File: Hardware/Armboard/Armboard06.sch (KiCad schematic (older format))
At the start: 7 parts

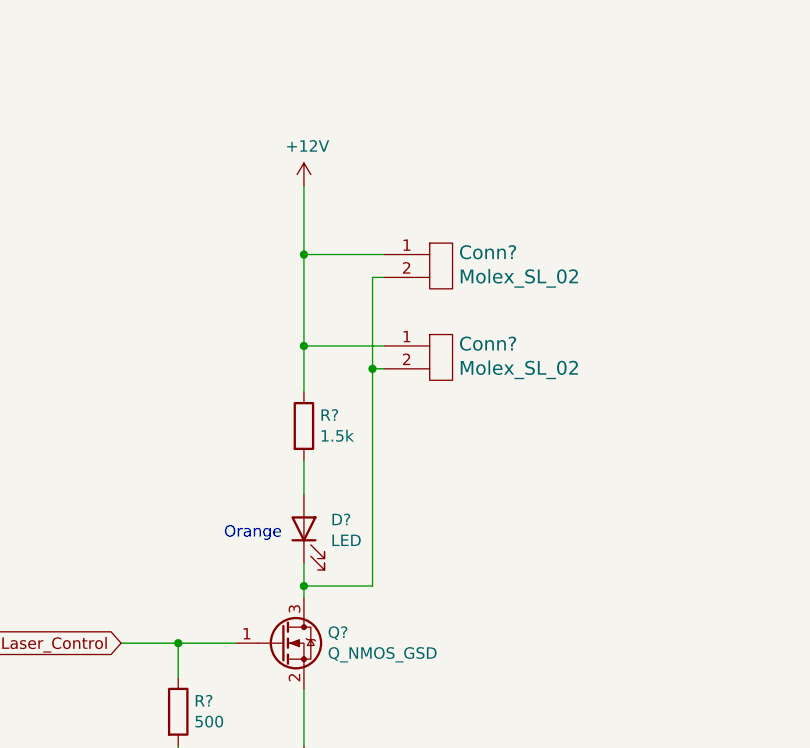
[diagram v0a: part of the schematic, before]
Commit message: Tiva Updates
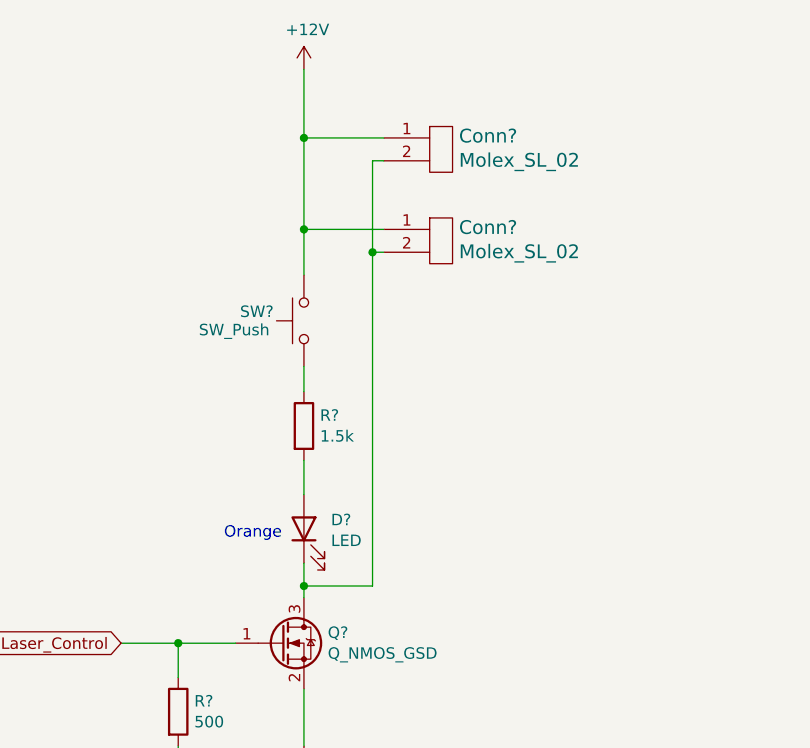
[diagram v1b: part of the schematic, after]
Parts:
- added SW?: SW_Push, symbol Switch:SW_Push
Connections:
- net +12V: now also SW?.2; no longer R?.1
- new net: R?.1, SW?.1
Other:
- moved on the sheet: Conn?
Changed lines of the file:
@@
 L Armboard-rescue:Molex_SL_02-MRDT_Connectors-Armboard-rescue Conn?
 U 1 1 5F795BD7
-P 5950 3100
-F 0 "Conn?" H 6078 3258 60  0000 L CNN
-F 1 "Molex_SL_02" H 6078 3152 60  0000 L CNN
-F 2 "" H 5950 3000 60  0001 C CNN
-F 3 "" H 5950 3000 60  0001 C CNN
-	1    5950 3100
+P 5950 2590
+F 0 "Conn?" H 6078 2748 60  0000 L CNN
+F 1 "Molex_SL_02" H 6078 2642 60  0000 L CNN
+F 2 "" H 5950 2490 60  0001 C CNN
+F 3 "" H 5950 2490 60  0001 C CNN
+	1    5950 2590
 	1    0    0    -1
 $EndComp
@@
 L Armboard-rescue:Molex_SL_02-MRDT_Connectors-Armboard-rescue Conn?
 U 1 1 5F795EEA
-P 5950 3500
-F 0 "Conn?" H 6078 3658 60  0000 L CNN
-F 1 "Molex_SL_02" H 6078 3552 60  0000 L CNN
-F 2 "" H 5950 3400 60  0001 C CNN
-F 3 "" H 5950 3400 60  0001 C CNN
-	1    5950 3500
+P 5950 2990
+F 0 "Conn?" H 6078 3148 60  0000 L CNN
+F 1 "Molex_SL_02" H 6078 3042 60  0000 L CNN
+F 2 "" H 5950 2890 60  0001 C CNN
+F 3 "" H 5950 2890 60  0001 C CNN
+	1    5950 2990
 	1    0    0    -1
 $EndComp
@@
 L power:+12V #PWR?
 U 1 1 5F795F80
-P 5400 2650
-F 0 "#PWR?" H 5400 2500 50  0001 C CNN
-F 1 "+12V" H 5415 2823 50  0000 C CNN
-F 2 "" H 5400 2650 50  0001 C CNN
-F 3 "" H 5400 2650 50  0001 C CNN
-	1    5400 2650
+P 5400 2140
+F 0 "#PWR?" H 5400 1990 50  0001 C CNN
+F 1 "+12V" H 5415 2313 50  0000 C CNN
+F 2 "" H 5400 2140 50  0001 C CNN
+F 3 "" H 5400 2140 50  0001 C CNN
+	1    5400 2140
 	1    0    0    -1
 $EndComp
@@
 	1    0    0    -1
 $EndComp
-Connection ~ 5400 2950
+Connection ~ 5400 2440
 Wire Wire Line
-	5400 2950 5400 2650
+	5400 2440 5400 2140
 $Comp
 L Device:Q_NMOS_GSD Q?
@@
 	5400 4450 5400 4400
 Wire Wire Line
-	5750 3450 5700 3450
+	5750 2940 5700 2940
 Wire Wire Line
-	5700 3050 5750 3050
+	5700 2540 5750 2540
 Wire Wire Line
-	5400 2950 5750 2950
+	5400 2440 5750 2440
 Wire Wire Line
-	5400 2950 5400 3350
+	5400 2440 5400 2840
 Wire Wire Line
-	5700 3050 5700 3450
+	5700 2540 5700 2940
 Wire Wire Line
-	5750 3350 5400 3350
-Connection ~ 5400 3350
+	5750 2840 5400 2840
+Connection ~ 5400 2840
 Wire Wire Line
-	5400 3350 5400 3550
-Wire Wire Line
-	5700 3450 5700 4400
+	5400 2840 5400 3040
 Wire Wire Line
 	5700 4400 5400 4400
-Connection ~ 5700 3450
+Connection ~ 5700 2940
 Connection ~ 5400 4400
 Wire Wire Line
@@
 Text Notes 6500 7150 0    157  ~ 31
 Laser Control
+$Comp
+L Switch:SW_Push SW?
+U 1 1 5F852FC5
+P 5400 3240
+F 0 "SW?" V 5440 3520 50  0000 R CNN
+F 1 "SW_Push" V 5360 3700 50  0000 R CNN
+F 2 "" H 5400 3440 50  0001 C CNN
+F 3 "~" H 5400 3440 50  0001 C CNN
+	1    5400 3240
+	0    -1   -1   0
+$EndComp
+Wire Wire Line
+	5400 3550 5400 3440
+Wire Wire Line
+	5700 2940 5700 4400
 $EndSCHEMATC
